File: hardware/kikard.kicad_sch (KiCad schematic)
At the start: 73 parts, among them Q1 WNM3013-3/TR, Q2 WNM3013-3/TR, SW1 K2-6639SP-C4SC-04, SW2 K2-6639SP-C4SC-04, SW3 K2-6639SP-C4SC-04, SW4 HX TS-1088-AR02016, U1 NRF52840-QIAA-R, U2 ST25R3916-AQWT, Y1 27MHz, Y2 32MHz, Y3 32.768kHz

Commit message: 7-16-25
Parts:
- U1: footprint NRF52840-QIAA-R:XCVR_NRF52840-QIAA-R -> extra-symbols-footprints:XCVR_NRF52840-QIAA-R
- U2: footprint ST25R3916-AQWT:QFN50P500X500X100-33N -> extra-symbols-footprints:QFN50P500X500X100-33N
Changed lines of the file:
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@@
 			)
 		)
-		(property "Footprint" "ST25R3916-AQWT:QFN50P500X500X100-33N"
+		(property "Footprint" "extra-symbols-footprints:QFN50P500X500X100-33N"
 			(at 402.59 455.93 0)
 			(effects
@@
 			)
 		)
-		(property "Footprint" "NRF52840-QIAA-R:XCVR_NRF52840-QIAA-R"
+		(property "Footprint" "extra-symbols-footprints:XCVR_NRF52840-QIAA-R"
 			(at 182.88 441.96 0)
 			(effects

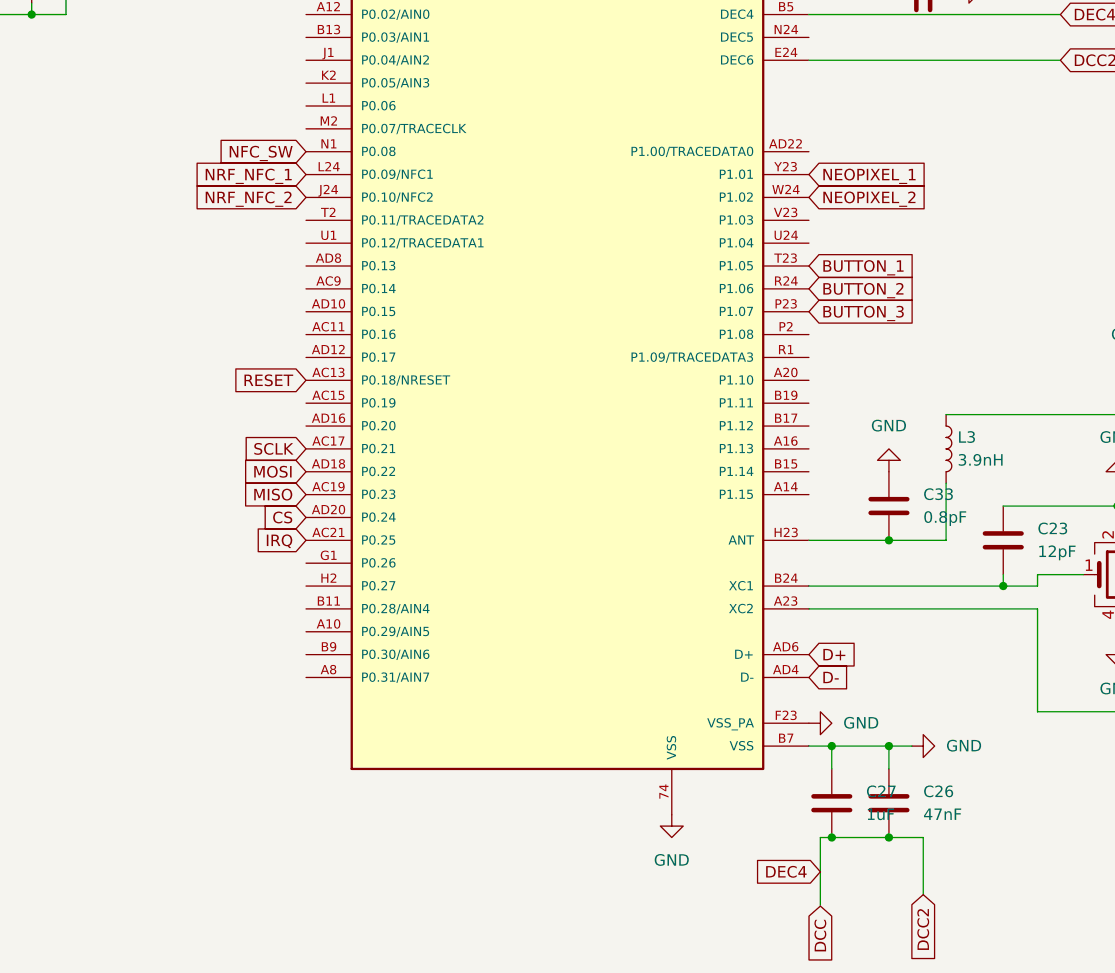
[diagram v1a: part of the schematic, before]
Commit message: 7-17-25
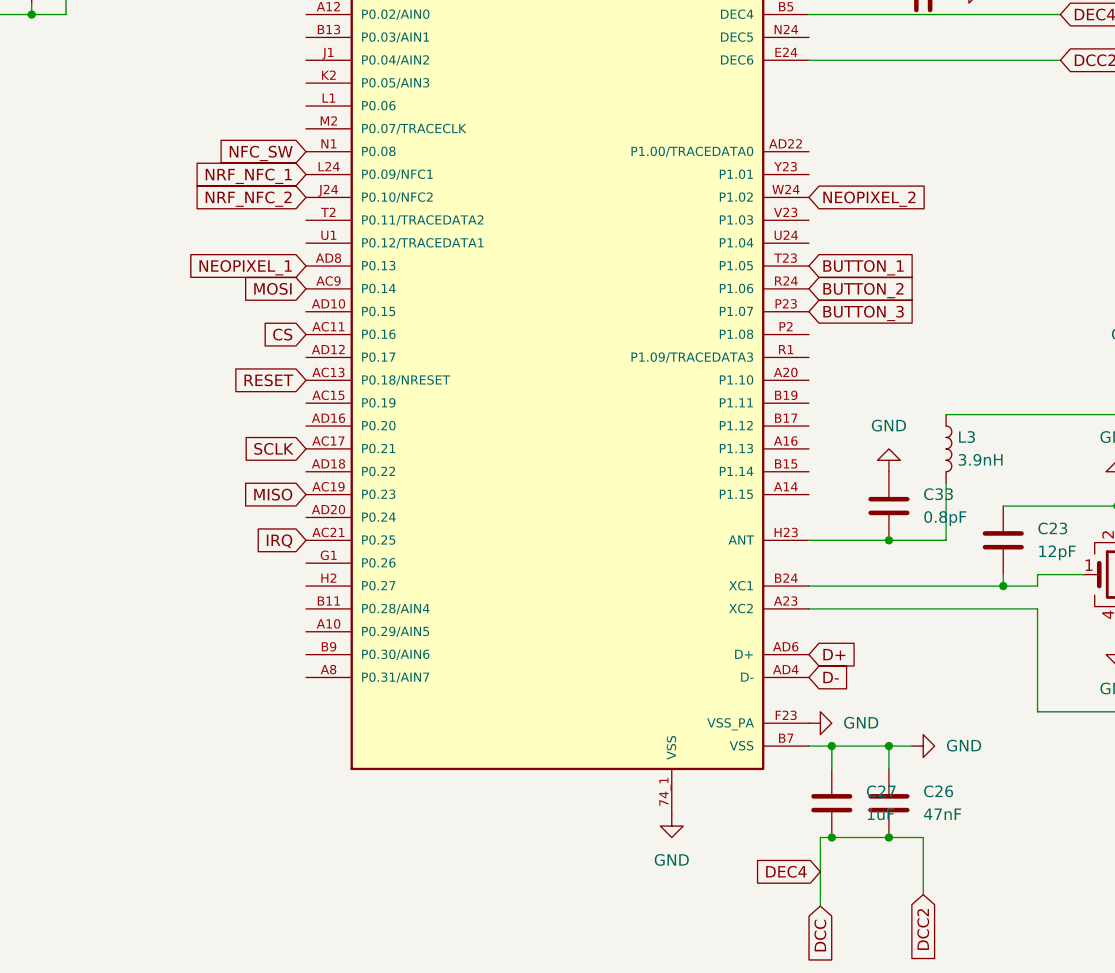
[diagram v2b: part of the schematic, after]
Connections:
- net CS: now also U1.AC11 (P0.16); no longer U1.AD20 (P0.24)
- net GND: now also U1.74_1 (VSS); no longer U1.74 (VSS)
- net MOSI: now also U1.AC9 (P0.14); no longer U1.AD18 (P0.22)
- net NEOPIXEL_1: now also U1.AD8 (P0.13); no longer U1.Y23 (P1.01)
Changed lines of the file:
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@@
 	(global_label "MOSI"
 		(shape input)
-		(at 154.94 464.82 180)
+		(at 154.94 444.5 180)
 		(fields_autoplaced yes)
 		(effects
@@
 		)
 		(property "Intersheetrefs" "${INTERSHEET_REFS}"
-			(at 147.3586 464.82 0)
+			(at 147.3586 444.5 0)
 			(effects
 				(font
@@
 	(global_label "NEOPIXEL_1"
 		(shape input)
-		(at 210.82 431.8 0)
+		(at 154.94 441.96 180)
 		(fields_autoplaced yes)
 		(effects
@@
 				(size 1.27 1.27)
 			)
-			(justify left)
+			(justify right)
 		)
 		(property "Intersheetrefs" "${INTERSHEET_REFS}"
-			(at 225.0537 431.8 0)
+			(at 140.7063 441.96 0)
 			(effects
 				(font
 					(size 1.27 1.27)
 				)
-				(justify left)
+				(justify right)
 				(hide yes)
 			)
@@
 	(global_label "CS"
 		(shape input)
-		(at 154.94 469.9 180)
+		(at 154.94 449.58 180)
 		(fields_autoplaced yes)
 		(effects
@@
 		)
 		(property "Intersheetrefs" "${INTERSHEET_REFS}"
-			(at 149.4753 469.9 0)
+			(at 149.4753 449.58 0)
 			(effects
 				(font
@@
 		(pin "A14"
 		)
-		(pin "74"
+		(pin "74_1"
 		)
 		(pin "G1"
